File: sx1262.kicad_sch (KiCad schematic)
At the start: 32 parts, among them U2 TPE4259-63, U3 SX1262IMLTRT, X2 S201632M10PF10PPM

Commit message: Routed buttons to MCU.
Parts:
- C25: footprint Capacitor_SMD:C_0603_1608Metric -> Capacitor_SMD:C_0402_1005Metric; LCSC C1622 -> C82219
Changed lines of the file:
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@@
-		(length 2.54)
-		(shape diamond)
-		(at 162.56 64.77 0)
-		(fields_autoplaced yes)
-		(effects
-			(font
-				(size 1.27 1.27)
-			)
-			(justify left bottom)
-		)
-		(property "Netclass" "LORA-RF"
-			(at 163.7665 62.23 0)
-			(effects
-				(font
-					(size 1.27 1.27)
-				)
-				(justify left)
-			)
-		)
-		(property "Component Class" ""
-			(at -50.8 -6.35 0)
-			(effects
-				(font
-					(size 1.27 1.27)
-					(italic yes)
-				)
-			)
-		)
-	)
-	(netclass_flag ""
 		(length 2.54)
 		(shape diamond)
@@
 			)
 		)
-		(property "Footprint" "Capacitor_SMD:C_0603_1608Metric"
+		(property "Footprint" "Capacitor_SMD:C_0402_1005Metric"
 			(at 152.4 68.58 0)
 			(effects
@@
 			)
 		)
-		(property "Datasheet" "https://jlcpcb.com/partdetail/1974-CL10B473KB8NNNC/C1622"
+		(property "Datasheet" "https://jlcpcb.com/partdetail/83376-0402B473K500NT/C82219"
 			(at 152.4 68.58 0)
 			(effects
@@
 			)
 		)
-		(property "LCSC" "C1622"
+		(property "LCSC" "C82219"
 			(at 152.4 68.58 90)
 			(effects

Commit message: Checked PCBA for JLCPCB.
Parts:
- C45: LCSC C318583 -> C41361091
- L8: LCSC C142213 -> C98003
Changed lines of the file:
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@@
 			)
 		)
-		(property "Datasheet" "https://jlcpcb.com/partdetail/299712-CL05C030BB5NNNC/C318583"
+		(property "Datasheet" "https://jlcpcb.com/partdetail/HRE-CGA0402C0G3R0C500GT/C41361091"
 			(at 179.07 68.58 0)
 			(effects
@@
 			)
 		)
-		(property "LCSC" "C318583"
+		(property "LCSC" "C41361091"
 			(at 179.07 68.58 90)
 			(effects
@@
 			)
 		)
-		(property "Datasheet" "https://jlcpcb.com/partdetail/ChilisinElec-CLH1005T_8N2J_SNP/C142213"
+		(property "Datasheet" "https://jlcpcb.com/partdetail/MurataElectronics-LQG15HS8N2J02D/C98003"
 			(at 260.35 86.36 0)
 			(effects
@@
 			)
 		)
-		(property "LCSC" "C142213"
+		(property "LCSC" "C98003"
 			(at 260.35 86.36 90)
 			(effects

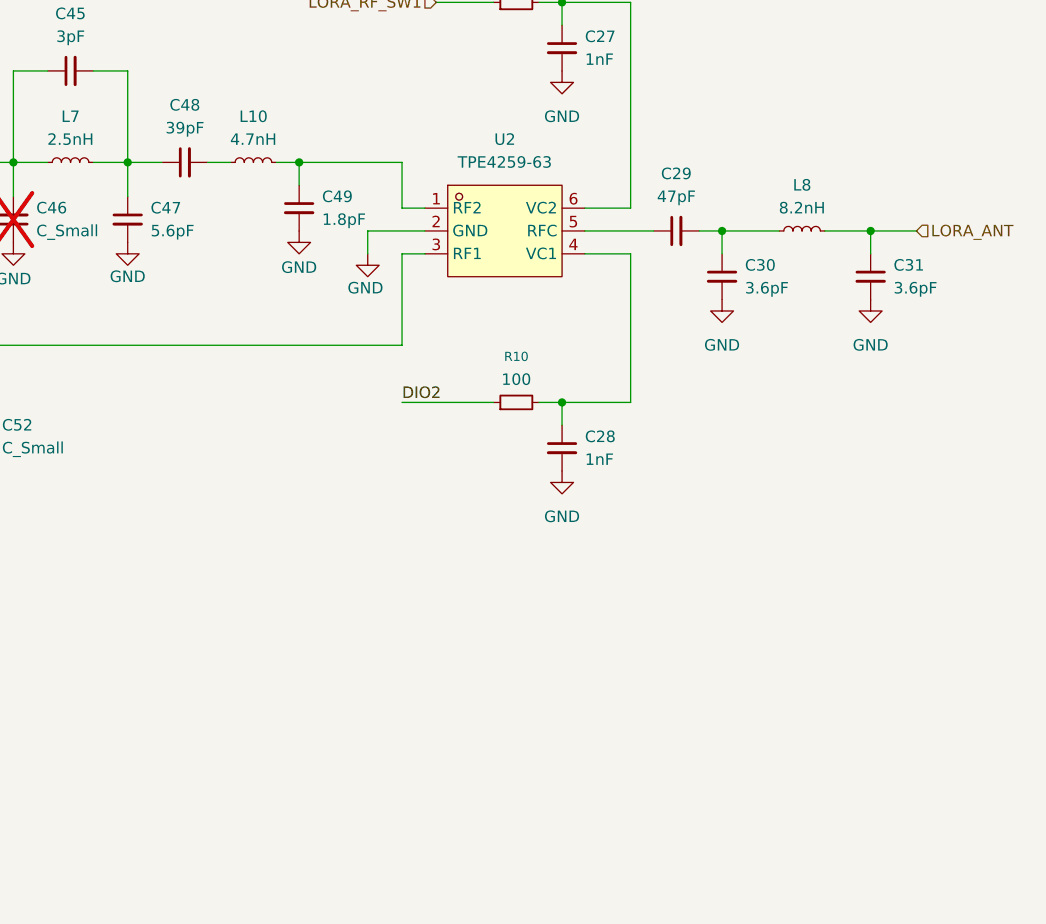
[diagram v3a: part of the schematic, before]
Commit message: Moved LoRa radio closer to antenna
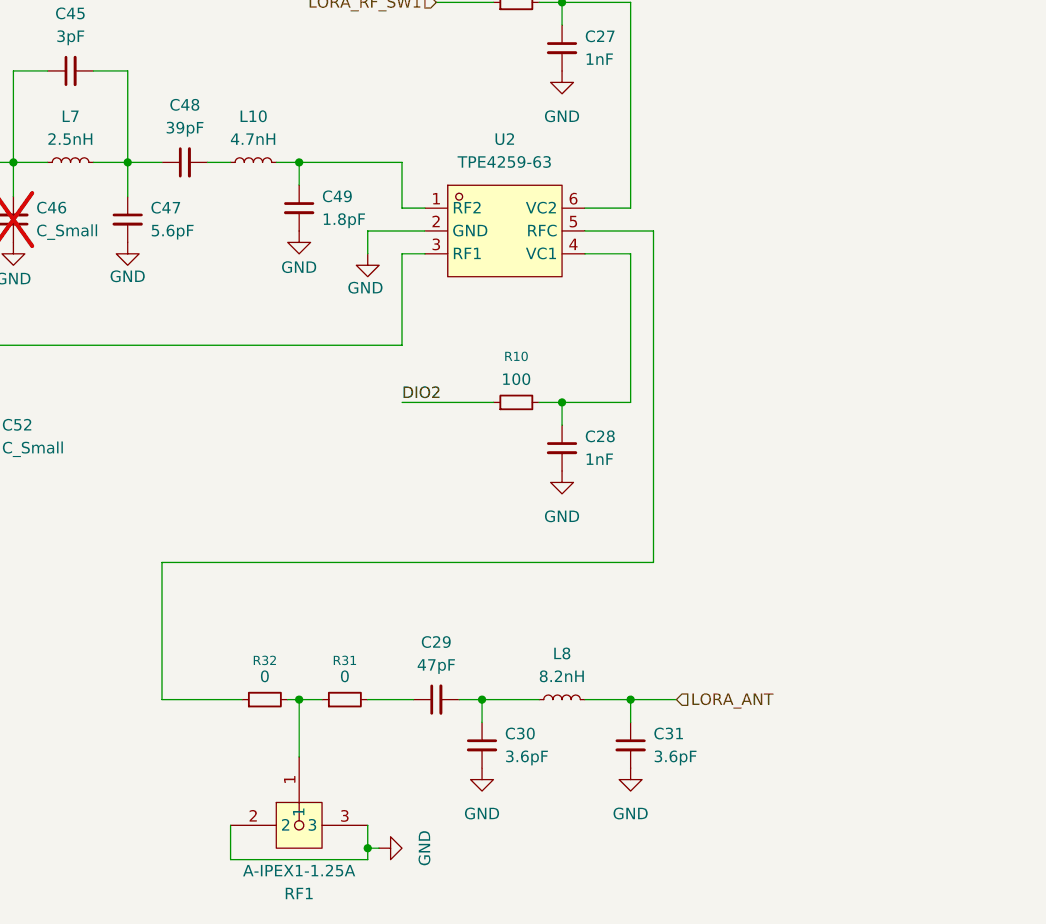
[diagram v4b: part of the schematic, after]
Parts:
- added R31, R32: 0, Resistor_SMD:R_0402_1005Metric, symbol Device:R_Small
- added RF1: A-IPEX1-1.25A, lcsc:IPEX-SMD_3P-L2.6-W2.6-LS3.0_RF1200001R, symbol lcsc:A-IPEX1-1.25A
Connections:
- net GND: now also RF1.2, RF1.3
- net at C29.1: now also R31.2; no longer U2.5 (RFC)
- new net: R31.1, R32.2, RF1.1
- new net: R32.1, U2.5 (RFC)
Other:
- moved on the sheet: C29, C30, C31, L8
